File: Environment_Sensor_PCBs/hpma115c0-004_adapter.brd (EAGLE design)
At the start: 26.7 x 17.8 mm, 10 parts, among them U1 BME680

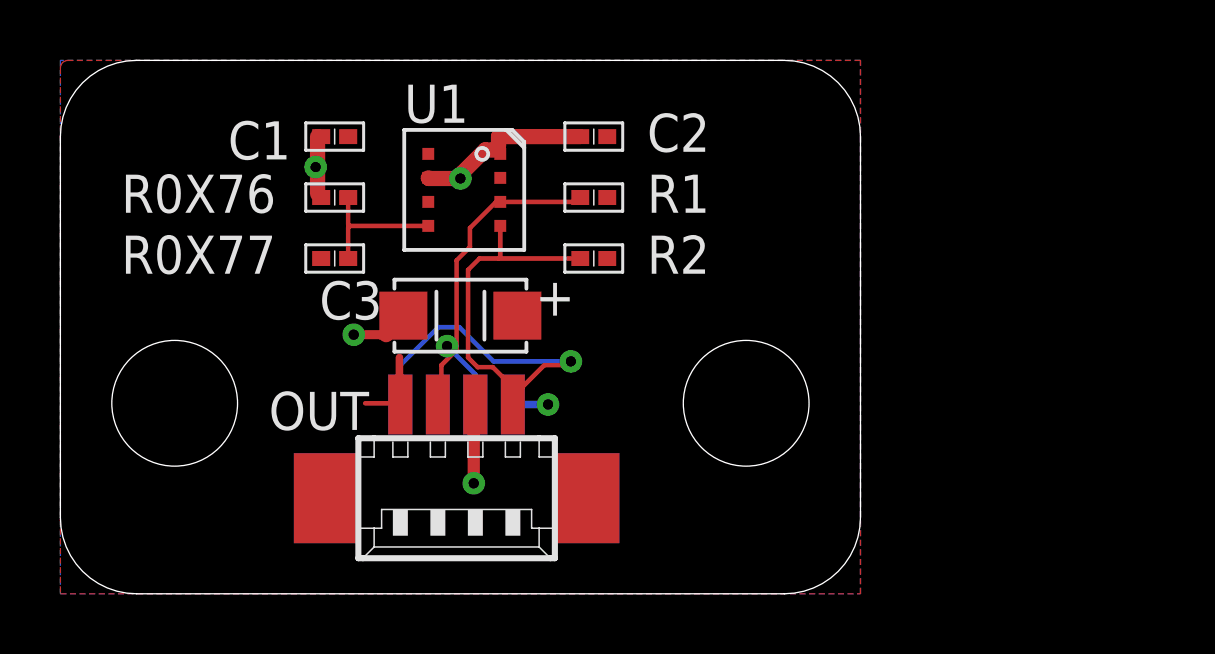
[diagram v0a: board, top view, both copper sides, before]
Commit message: Adding most recent boards
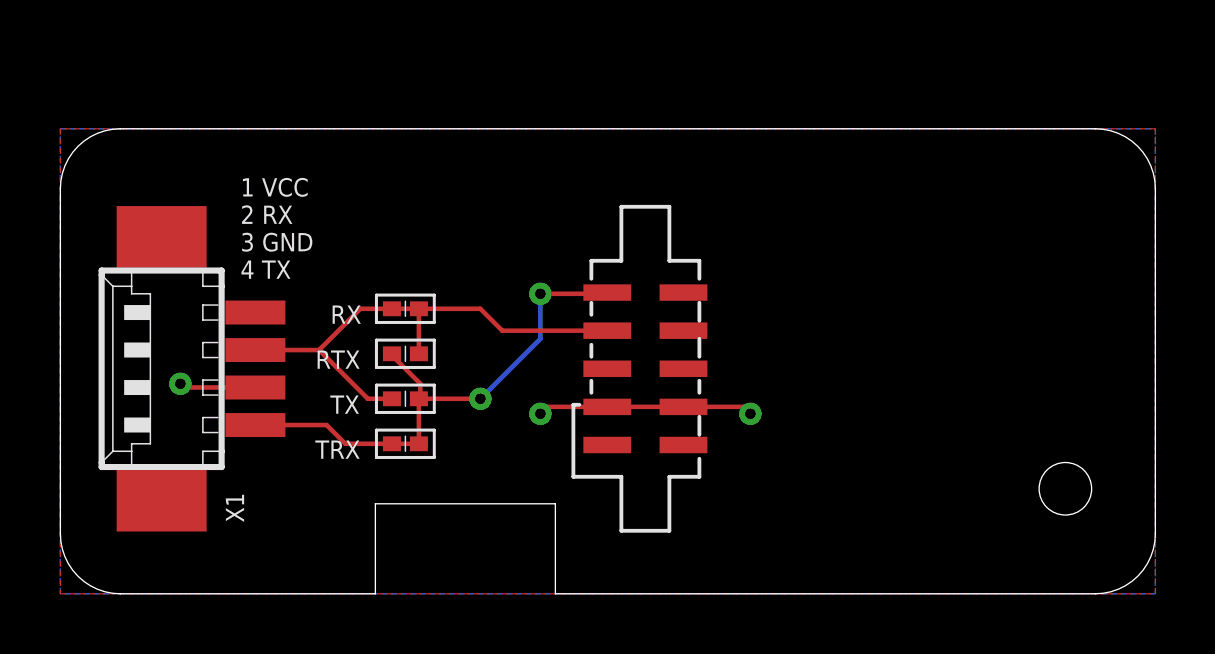
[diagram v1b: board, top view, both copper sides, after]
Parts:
- removed C1, C2: 100nF, daneagle_db8.0:SMD_0402
- removed C3: 10uF, daneagle_db8.0:CAP_POL_1206
- removed IN, OUT: 53261-04, con-molex:53261-04
- removed R0X76: 0r, daneagle_db8.0:SMD_0402
- removed R0X77: dnp, daneagle_db8.0:SMD_0402
- removed R1, R2: 4k7, daneagle_db8.0:SMD_0402
- removed U1: BME680, daneagle_db8.0:BOSCH_LGA8
- added CON1: HEADER_5X2_SFM-105-02-H-D, daneagle_db8.0:HEADER_5X2_1.27X1.27_SMD_SAMTEK
- added RTX, RX, TRX, TX: DNP, daneagle_db8.0:SMD_0402
- added X1: 53261-04, con-molex:53261-04
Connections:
- removed net 3V3: C1.P$1, C2.P$1, C3.P, IN.1, OUT.1, R0X77.P$1, R1.P$2, R2.P$2, U1.P$2, U1.P$6, U1.P$8
- removed net ADDR: R0X76.P$2, R0X77.P$2, U1.P$5
- removed net SCL: IN.4, OUT.4, R2.P$1, U1.P$4
- removed net SDA: IN.2, OUT.2, R1.P$1, U1.P$3
- new net RX: CON1.P$7, RTX.P$2, RX.P$1, RX.P$2, TX.P$1, X1.2
- new net TX: CON1.P$9, RTX.P$1, TRX.P$1, TRX.P$2, TX.P$2, X1.4
- new net VCC: CON1.P$2, X1.1
- net GND: now also CON1.P$3, CON1.P$4, X1.3; no longer C1.P$2, C2.P$2, C3.N, IN.3, OUT.3, R0X76.P$1, U1.P$1, U1.P$7
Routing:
- net SCL: track 21.4 -> 0.00 mm, vias 1 -> 0
- net TX: track 0.00 -> 17.7 mm, vias 0 -> 2
- net RX: track 0.00 -> 17.2 mm
- net SDA: track 13.1 -> 0.00 mm, vias 1 -> 0
- net GND: track 14.5 -> 9.74 mm, vias 4 -> 3
- net ADDR: track 4.69 -> 0.00 mm
- net 3V3: track 3.98 -> 0.00 mm, vias 1 -> 0
- added copper zone on layer 1, net VCC
- removed copper zone on layer 1, net 3V3
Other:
- board size 26.7 x 17.8 mm -> 36.5 x 15.5 mm
- board text added: "0,15.5"
- board text added: "1 VCC 2 RX 3 GND 4 TX"
- board text added: "10.5,0"
- board text added: "16.5,0"
- board text added: "16.5,3"
- board text added: "19.5x7.5"
- board text added: "33.5,3.5"
- board text added: "36.5,0"
- board text added: "36.5,15.5"
- board text added: "4,7.5"
- board text added: "HPMA115C0 CONN_BRD DAN NEAR 08-17-2020"
- board text removed: "BME680-GAS AQ/ BARO/TEMP/HUMID DAN NEAR Rev 3 2020-07-22"
